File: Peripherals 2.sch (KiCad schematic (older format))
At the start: 1 part, among them U1 IMX6UL_BGA289

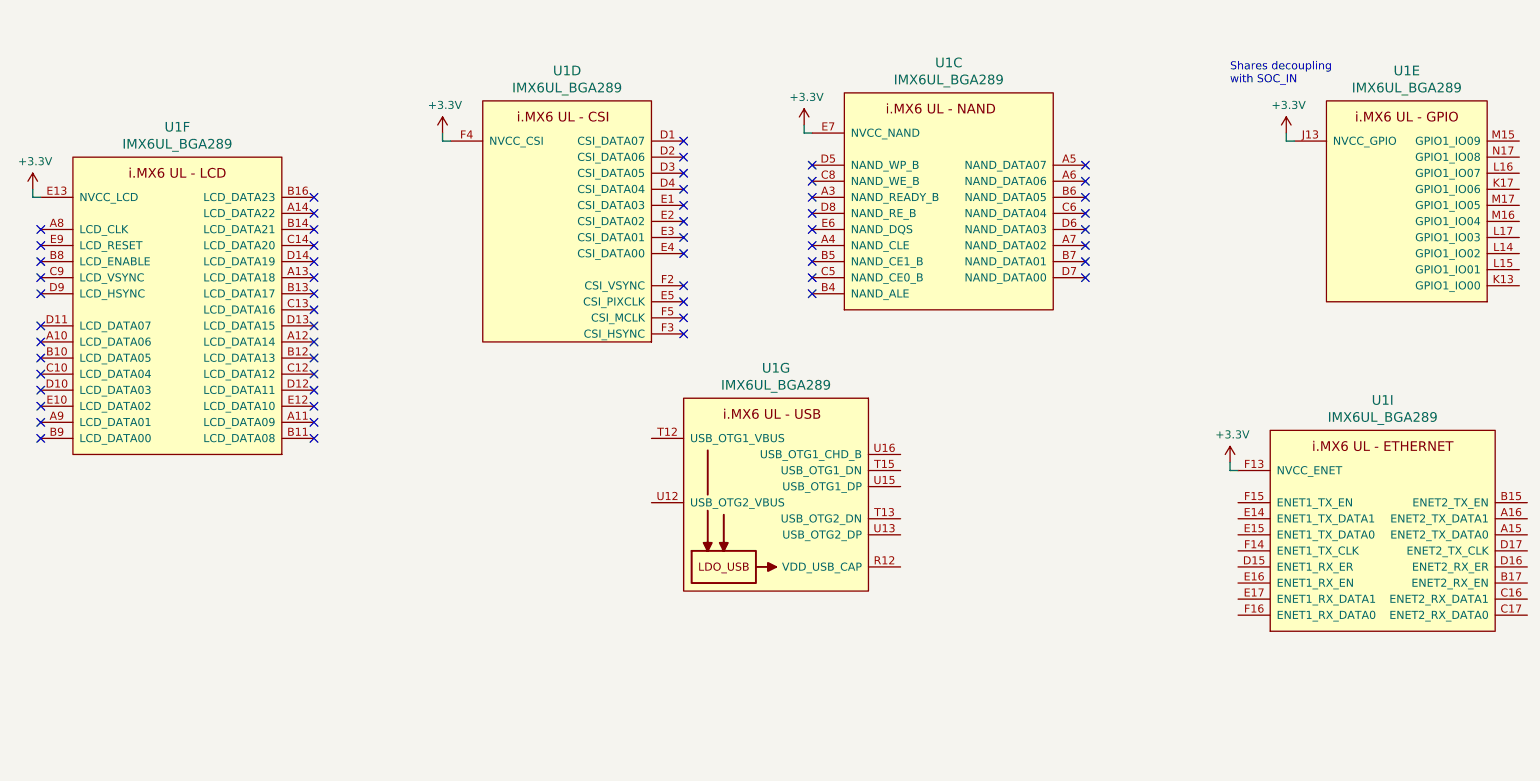
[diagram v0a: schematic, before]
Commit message: Finished first version of board
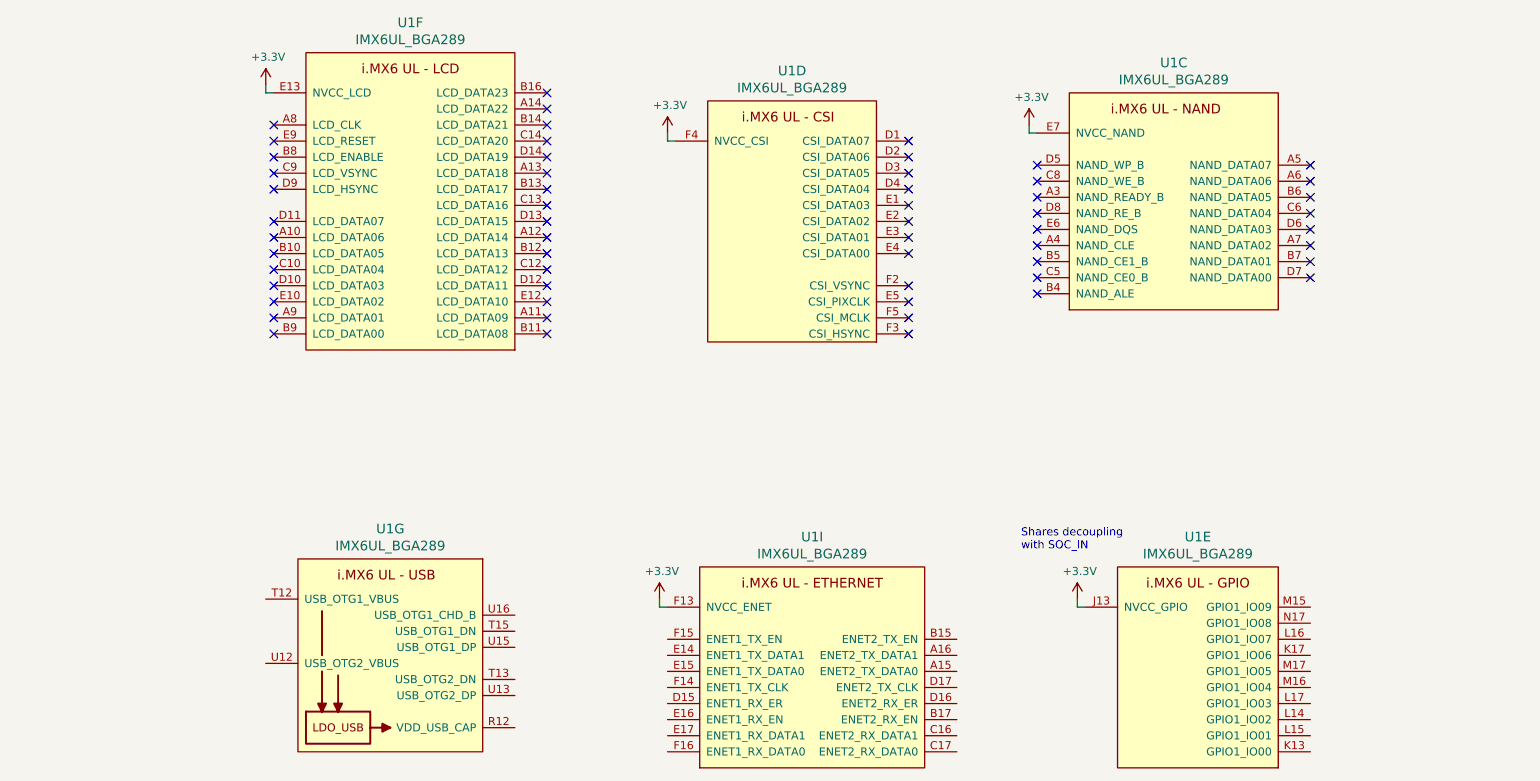
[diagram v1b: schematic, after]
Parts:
- U1: LCSC (none) -> C414042
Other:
- moved on the sheet: U1C, U1D, U1E, U1F, U1G, U1I
